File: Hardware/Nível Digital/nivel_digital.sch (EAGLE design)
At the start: 9 parts

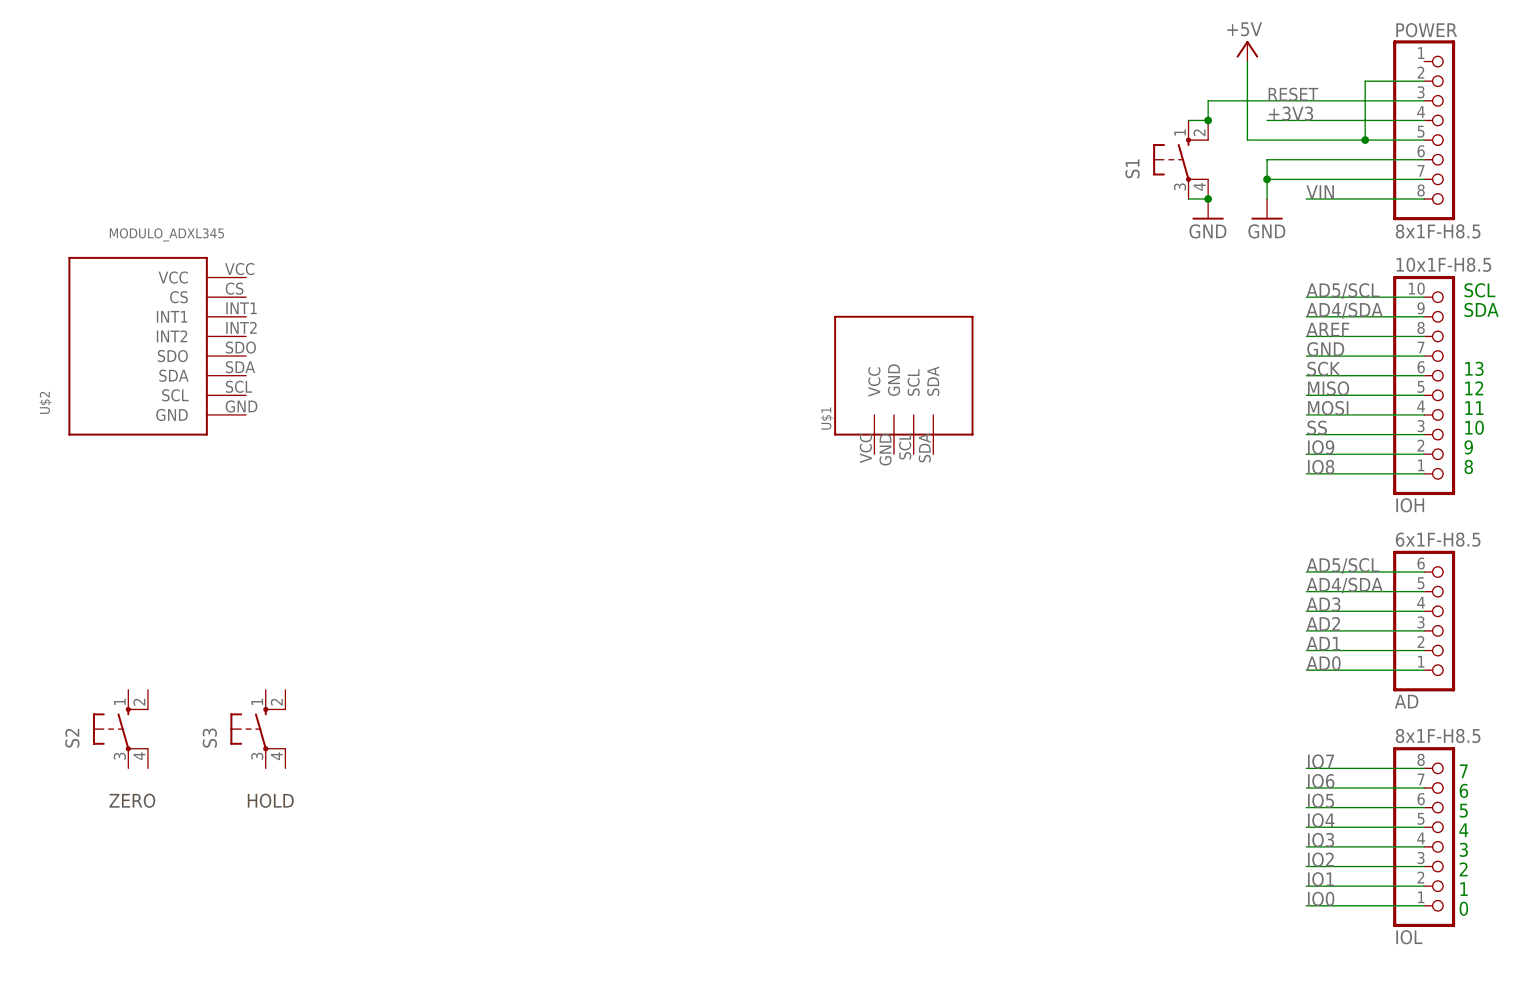
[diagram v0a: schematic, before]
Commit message: Botão range adicionado
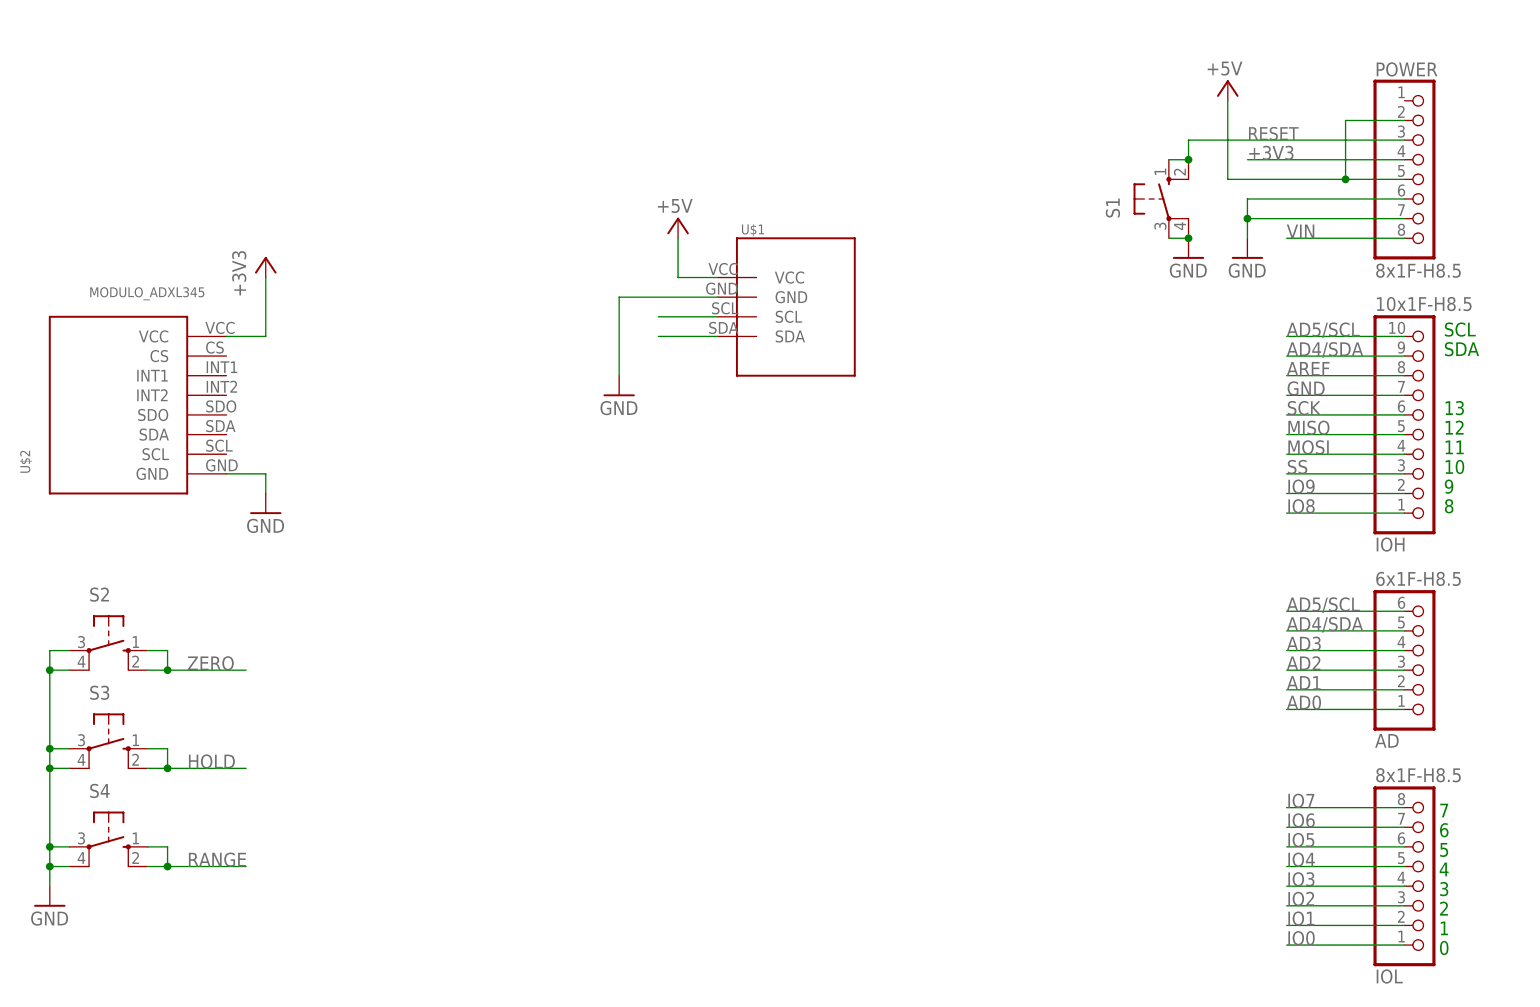
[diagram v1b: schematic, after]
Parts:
- added S4: (no value), GEAP:10-XXPUSH-BUTTON-5MM
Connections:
- new net HOLD: S3.S, S3.S1
- new net N$1: U$1.SCL
- new net N$2: U$1.SDA
- new net RANGE: S4.S, S4.S1
- new net ZERO: S2.S, S2.S1
- net +3V3: now also U$2.VCC
- net +5V: now also U$1.VCC
- net GND: now also S2.P, S2.P1, S3.P, S3.P1, S4.P, S4.P1, U$1.GND, U$2.GND
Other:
- note removed: "HOLD"
- note removed: "ZERO"
- moved on the sheet: AD, IOH, IOL, POWER, S1, S2, S3, U$1, U$2
